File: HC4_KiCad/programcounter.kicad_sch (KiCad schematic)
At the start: 20 parts, among them IC13 74HC161, IC14 74HC161, IC15 74HC161

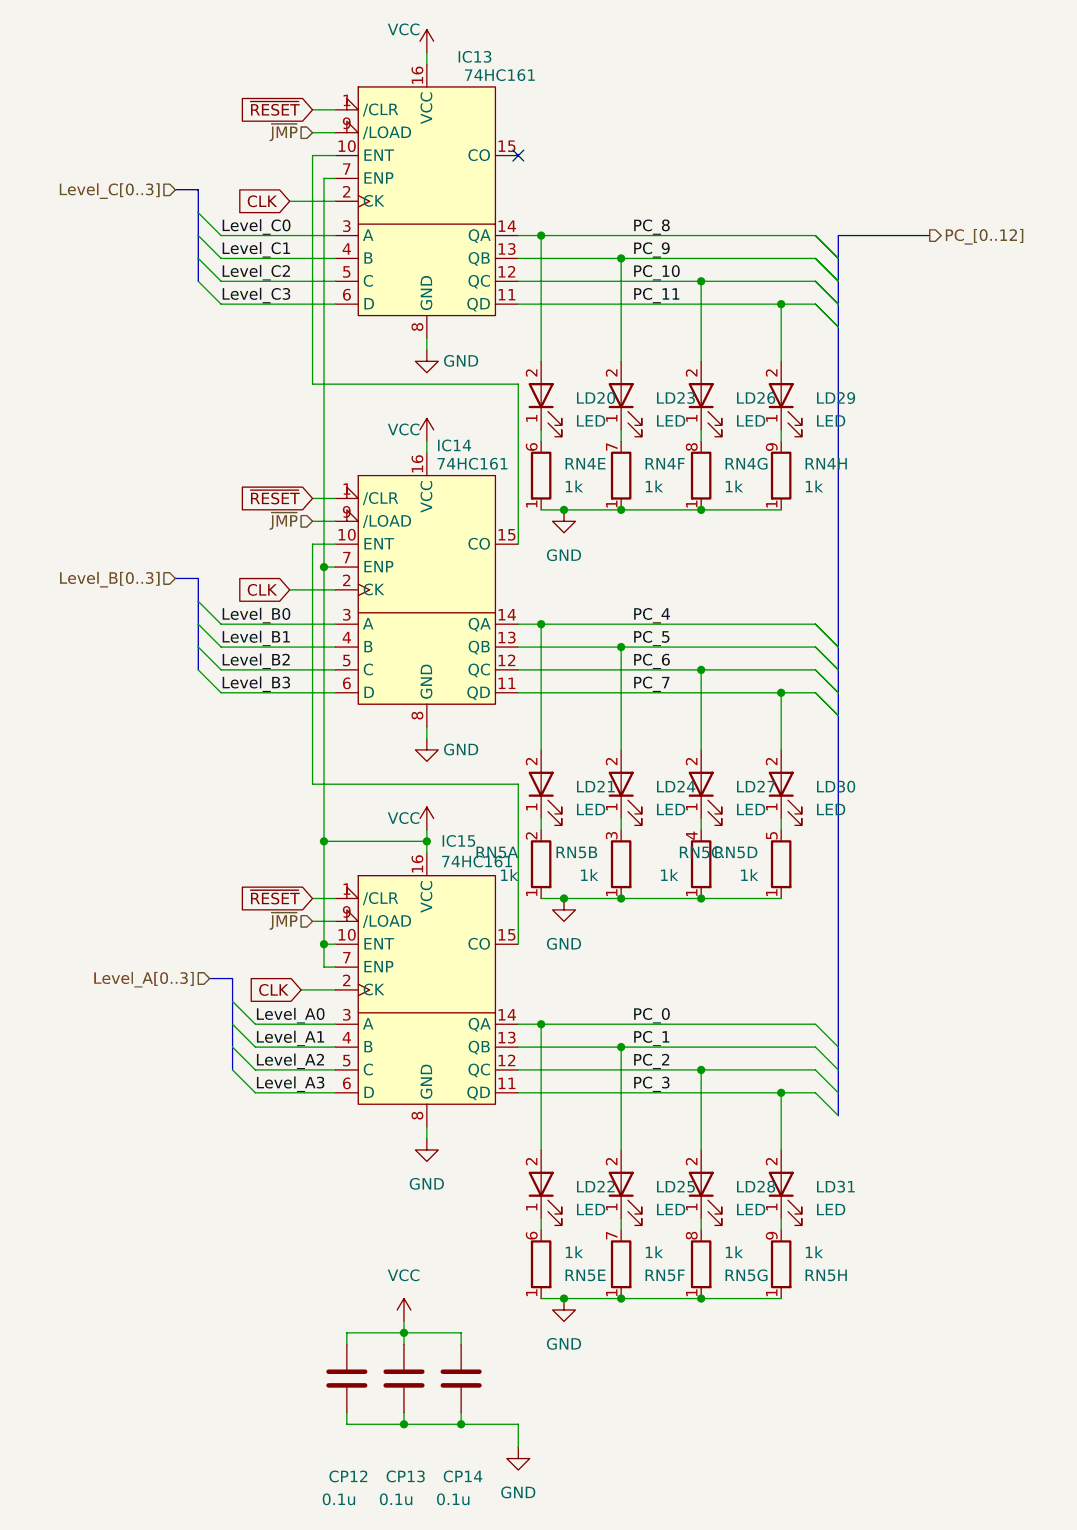
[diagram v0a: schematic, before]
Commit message: 基板ぬ
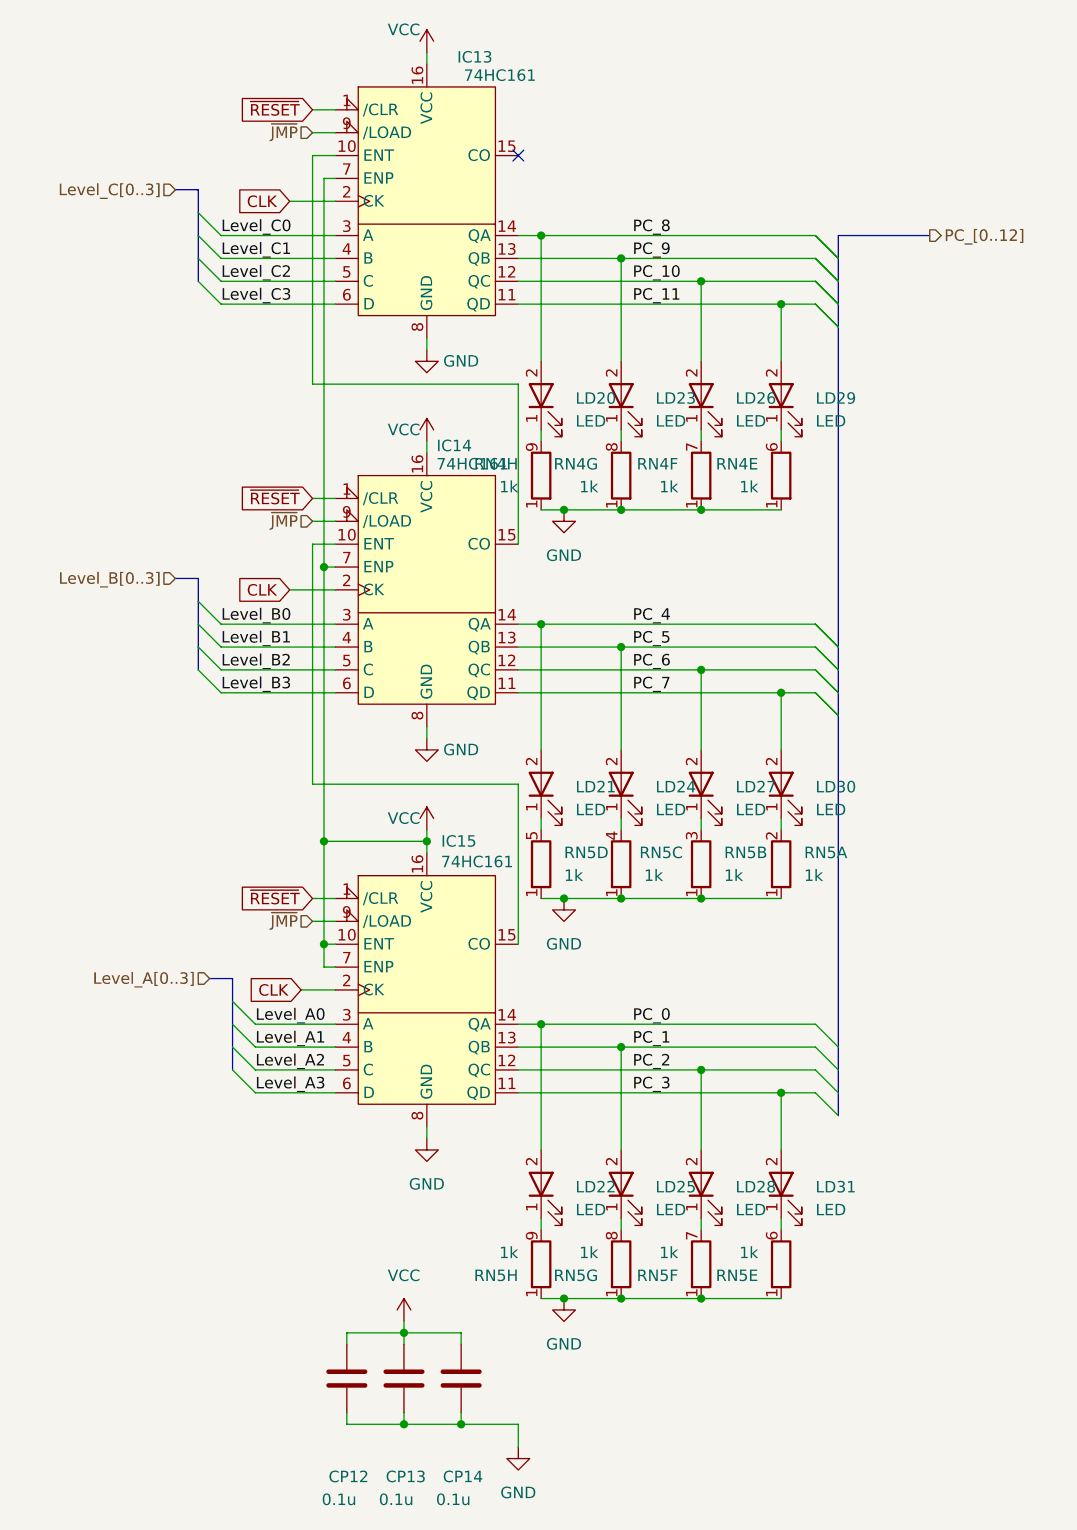
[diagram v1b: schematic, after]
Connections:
- net at LD30.1 (K): now also RN5.2 (R1.2); no longer RN5.5 (R4.2)
- net at RN5.3 (R2.2): now also LD27.1 (K); no longer LD24.1 (K)
- net at LD29.1 (K): now also RN4.6 (R5.2); no longer RN4.9 (R8.2)
- net at RN5.4 (R3.2): now also LD24.1 (K); no longer LD27.1 (K)
- net at RN5.7 (R6.2): now also LD28.1 (K); no longer LD25.1 (K)
- net at LD20.1 (K): now also RN4.9 (R8.2); no longer RN4.6 (R5.2)
- net at RN5.8 (R7.2): now also LD25.1 (K); no longer LD28.1 (K)
- net at LD21.1 (K): now also RN5.5 (R4.2); no longer RN5.2 (R1.2)
- net at RN5.9 (R8.2): now also LD22.1 (K); no longer LD31.1 (K)
- net at LD23.1 (K): now also RN4.8 (R7.2); no longer RN4.7 (R6.2)
- net at RN5.6 (R5.2): now also LD31.1 (K); no longer LD22.1 (K)
- net at LD26.1 (K): now also RN4.7 (R6.2); no longer RN4.8 (R7.2)
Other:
- moved on the sheet: RN4E, RN4F, RN4G, RN4H, RN5A, RN5B, RN5C, RN5D, RN5E, RN5F, RN5G, RN5H
